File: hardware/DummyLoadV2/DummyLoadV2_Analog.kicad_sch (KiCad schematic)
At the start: 49 parts, among them J2 Conn_01x05, J5 Power, J8 Digital, Q1 FQP30N06L, Q2 2N7000, Q5 2N7000, U1 MAX4167, U2 LM4040-4.1, U3 MCP3302, U7 L78L05_TO92, U8 MCP4922

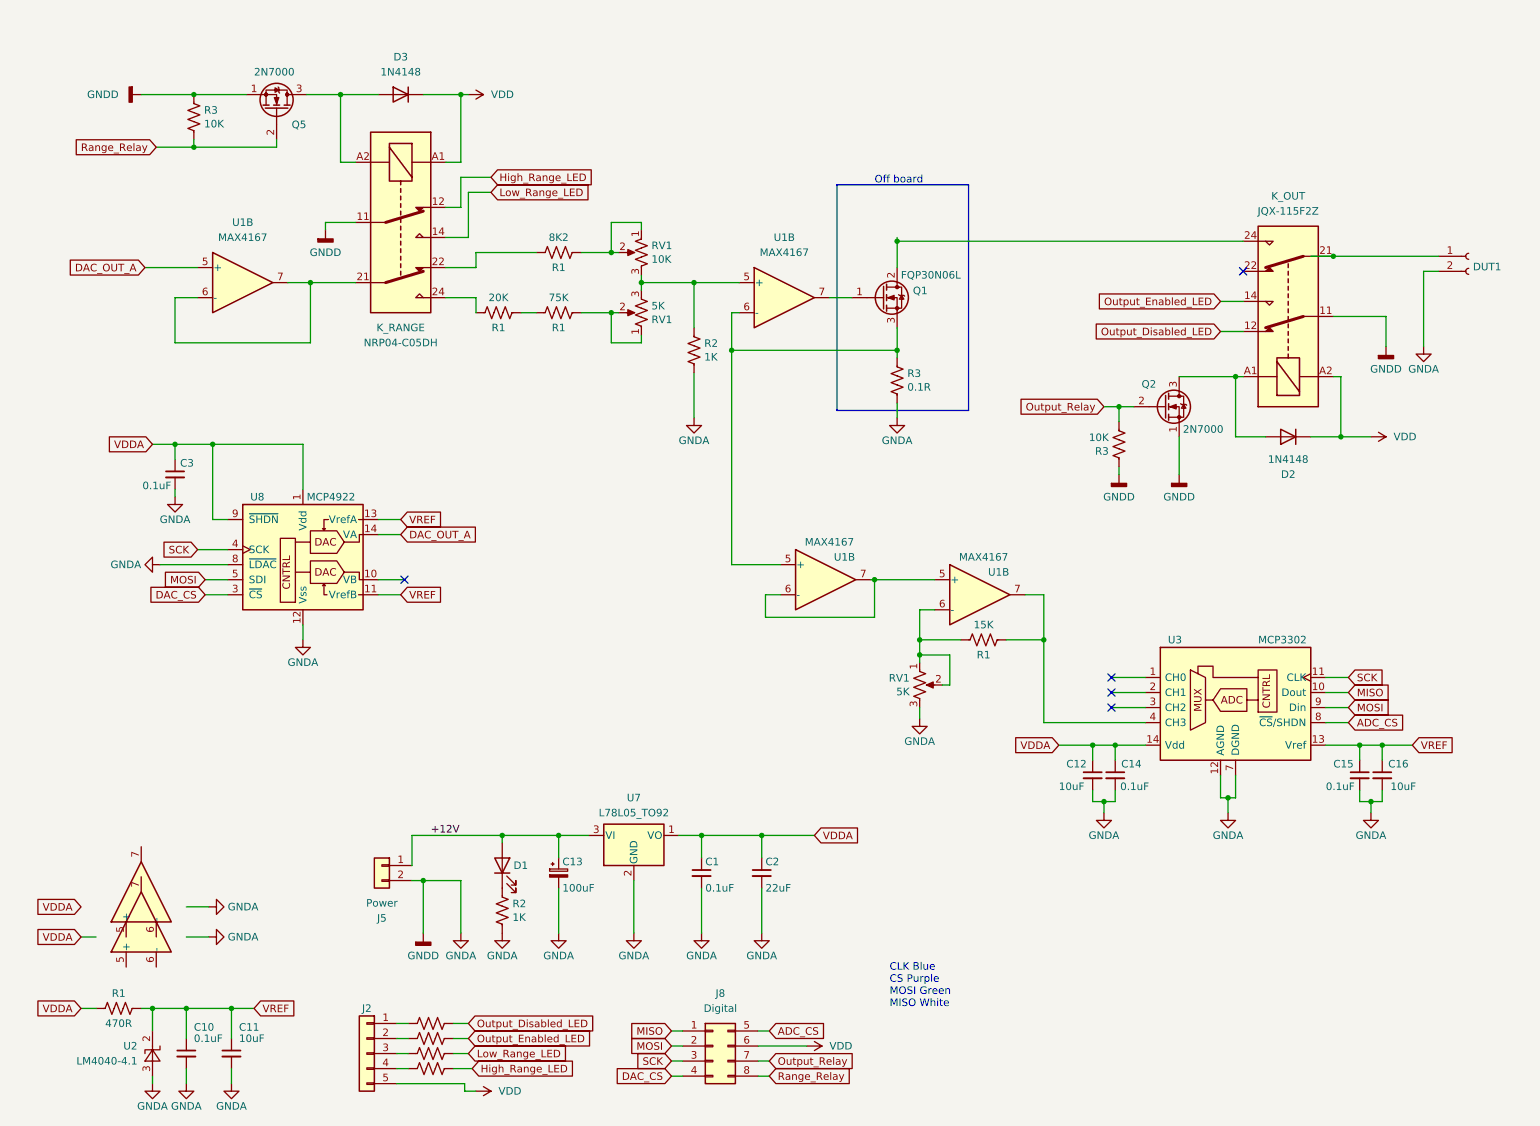
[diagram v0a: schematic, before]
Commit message: Updated schematic
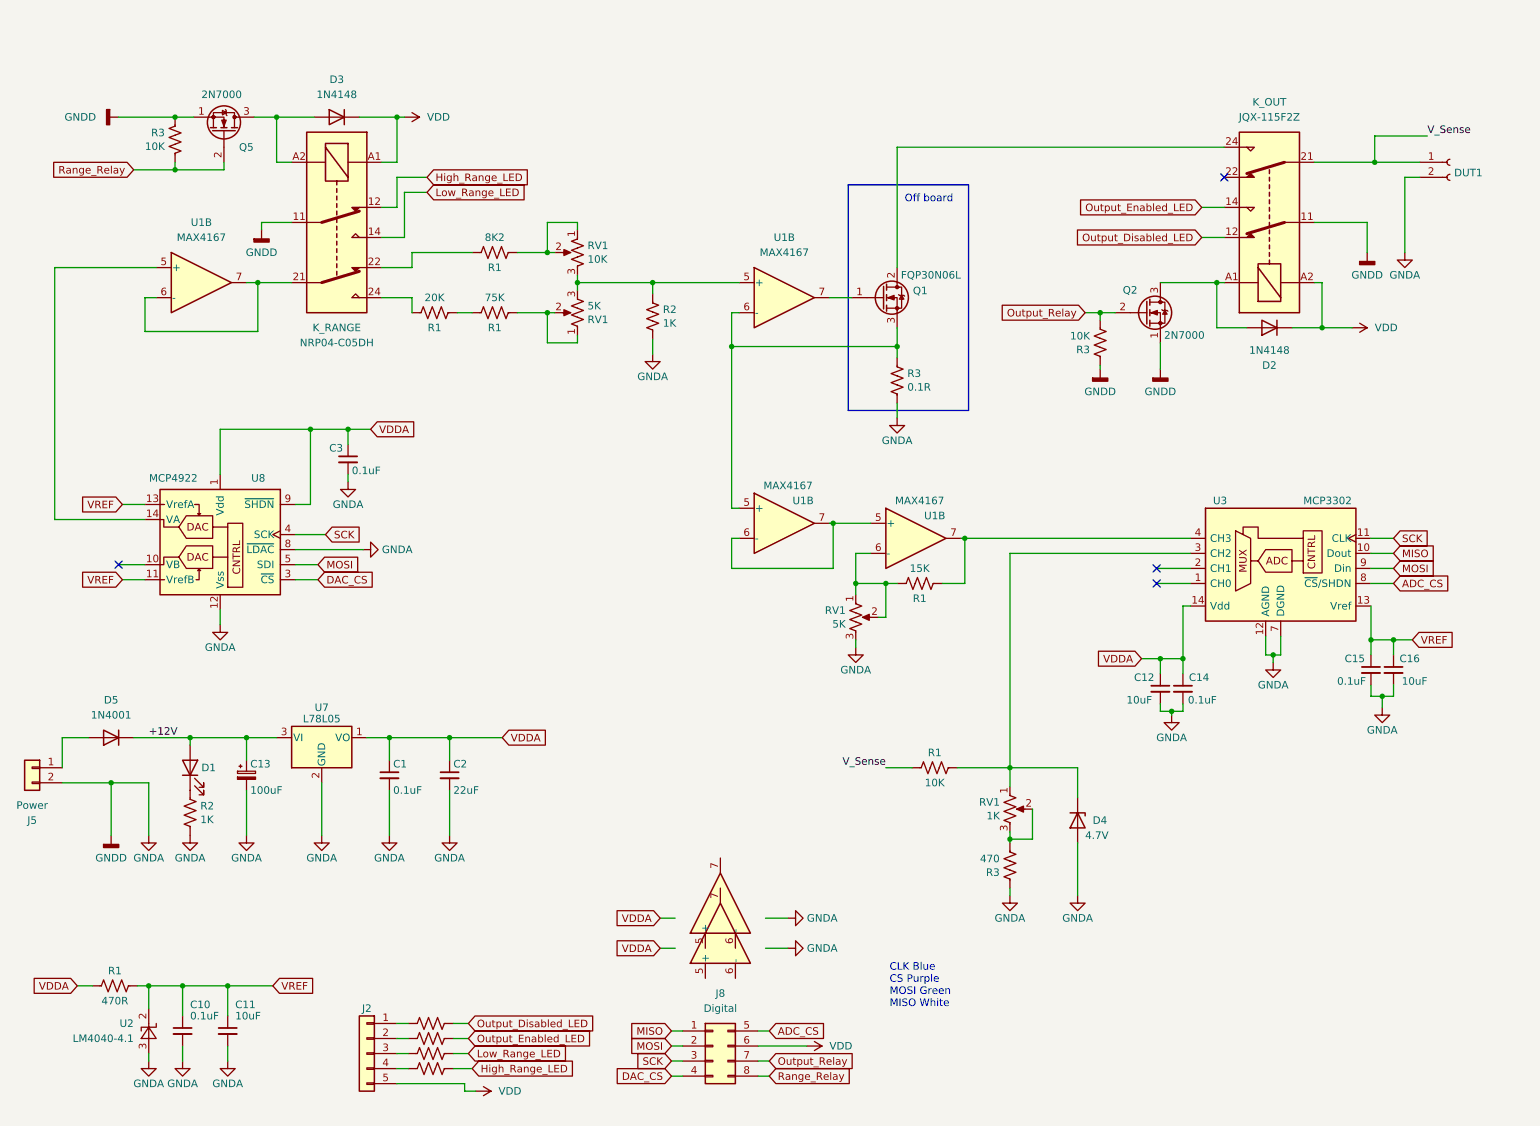
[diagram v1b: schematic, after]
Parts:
- added D4: 4.7V, symbol Device:D_Zener
- added D5: 1N4001, Diode_THT:D_DO-41_SOD81_P10.16mm_Horizontal, symbol Diode:1N4001
- added R1: 10K, symbol Device:R_US
- added R3: 470, symbol Device:R_US
- added RV1: 1K, symbol BasicDummyLoad-rescue:R_POT_US-Device
- U7: value L78L05_TO92 -> L78L05
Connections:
- net +12V: now also D5.1 (K); no longer J5.1 (Pin_1)
- net GNDA: now also D4.2 (A), R3.2
- net V_Sense: now reaches DUT1.1 (Pin_1), K_OUT.21
- net V_Sense: now also R1.2
- net at U3.3 (CH2): now also D4.1 (K), R1.1, RV1.1
- net DAC_OUT_A: no longer names the net of U1.5 (+), U8.14 (VA)
- new net: R3.1, RV1.2, RV1.3
- new net: D5.2 (A), J5.1 (Pin_1)
- no-connect marks 5 -> 4
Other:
- moved on the sheet: C1, C10, C11, C12, C13, C14, C15, C16, C2, C3, D1, D2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

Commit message: Updated schematic
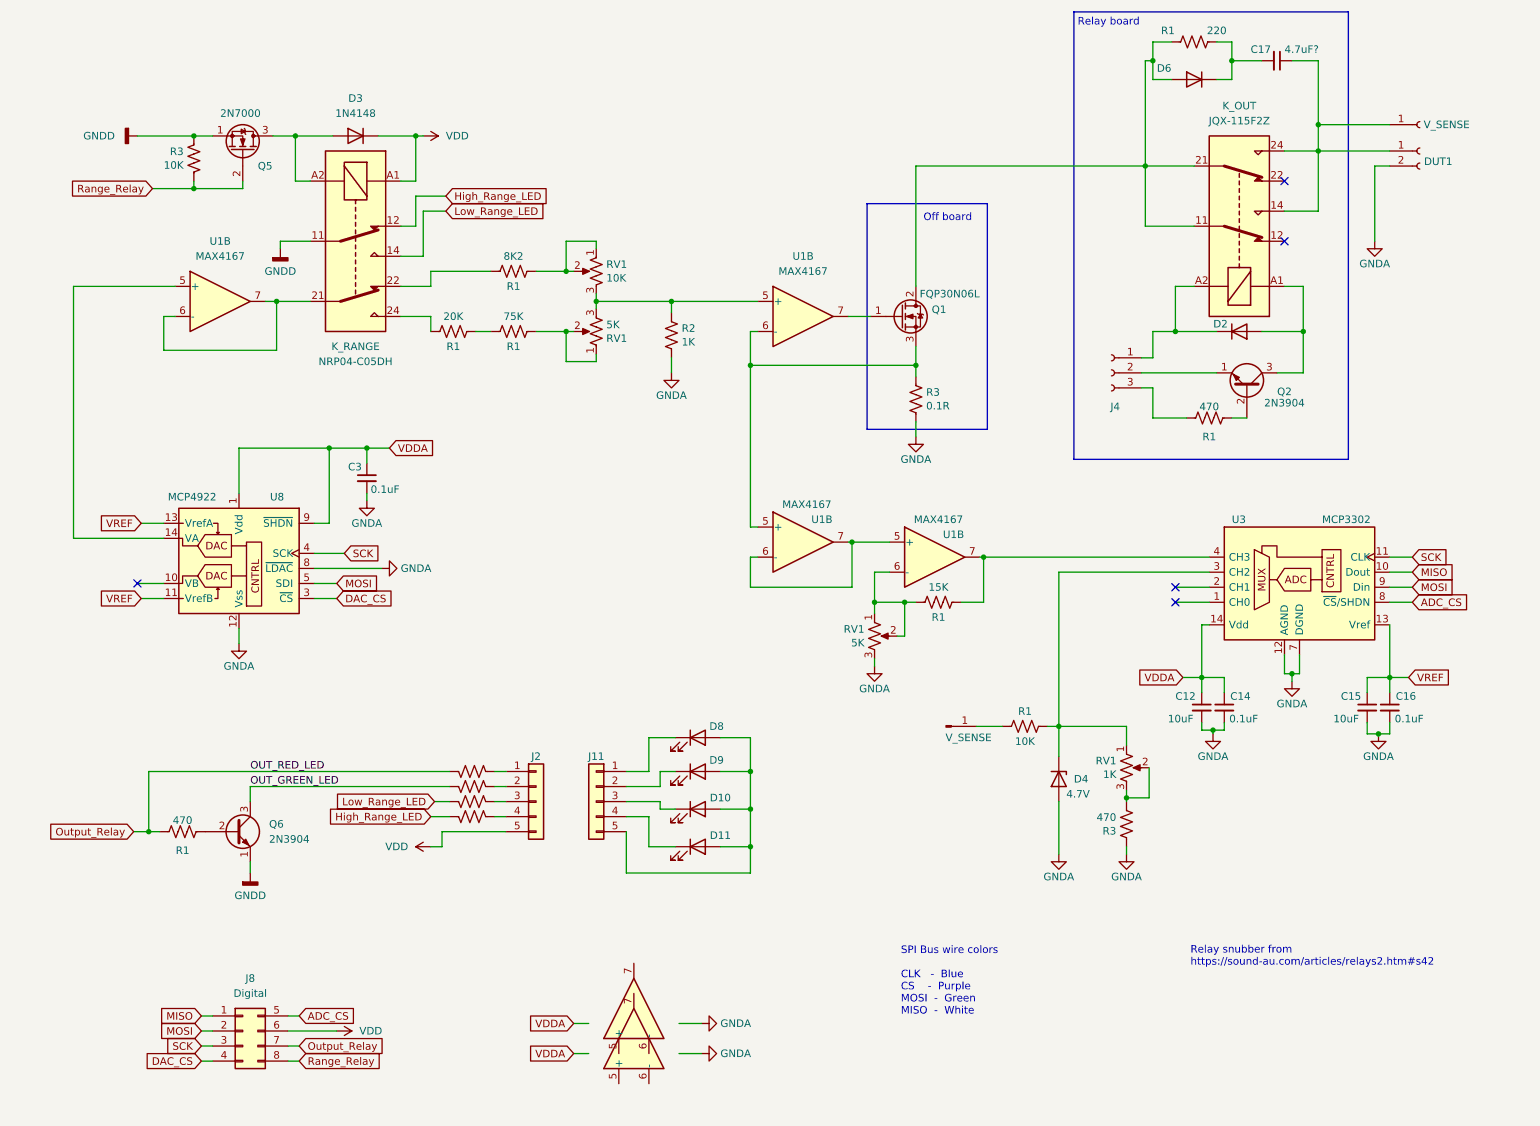
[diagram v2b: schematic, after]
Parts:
- removed C1, C10: 0.1uF, symbol Device:C_Small
- removed C11: 10uF, symbol Device:C_Small
- removed C13: 100uF, symbol Device:C_Polarized_Small
- removed C2: 22uF, symbol Device:C_Small
- removed D1: LED, symbol Device:LED
- removed D5: 1N4001, Diode_THT:D_DO-41_SOD81_P10.16mm_Horizontal, symbol Diode:1N4001
- removed J5: Power, symbol Connector_Generic:Conn_01x02
- removed Q2: 2N7000, Package_TO_SOT_THT:TO-92_Inline, symbol Transistor_FET:2N7000
- removed R1: 470R, symbol Device:R_US
- removed R2: 1K, symbol Device:R_US
- removed R3: 10K, symbol Device:R_US
- removed U2: LM4040-4.1, Package_TO_SOT_THT:TO-92_Inline, symbol Reference_Voltage:LM4040LP-4.1
- removed U7: L78L05, Package_TO_SOT_THT:TO-92_Inline, symbol Regulator_Linear:L78L05_TO92
- added C17: 4.7uF?, symbol Device:C_Small
- added D10, D11, D8, D9: LED, symbol Device:LED
- added D6: 1N4148, Diode_THT:D_DO-35_SOD27_P7.62mm_Horizontal, symbol Diode:1N4148
- added J11: Conn_01x05, symbol Connector_Generic:Conn_01x05
- added J4: Conn_01x03_Socket, symbol Connector:Conn_01x03_Socket
- added Q2, Q6: 2N3904, Package_TO_SOT_THT:TO-92_Inline, symbol Transistor_BJT:2N3904
- added R1 (x2): 470, symbol Device:R_US
- added R1: 220, symbol Device:R_US
- added V_SENSE: Conn_01x01_Pin, symbol Connector:Conn_01x01_Pin
- added V_SENSE: Conn_01x01_Socket, symbol Connector:Conn_01x01_Socket
- C15: value 0.1uF -> 10uF
- C16: value 10uF -> 0.1uF
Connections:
- net GNDA: no longer K_OUT.11, K_RANGE.11, Q5.1 (S), R3.2
- net Output_Relay: now also R1.1, R1.1
- net VDD: no longer D2.1 (K), K_OUT.A2
- net at D2.2 (A), K_OUT.A1: now also Q2.3 (C)
- net at K_OUT.24: now also DUT1.1 (Pin_1), K_OUT.14, C17.1, V_SENSE.1 (Pin_1); no longer Q1.2 (D)
- net Output_Disabled_LED: no longer names the net of K_OUT.12
- net Output_Disabled_LED: no longer R1.1
- net Output_Enabled_LED renamed OUT_GREEN_LED
- net OUT_GREEN_LED: now also Q6.3 (C); no longer K_OUT.14
- removed net V_Sense: DUT1.1 (Pin_1), K_OUT.21, R1.2
- new net: D8.1 (K), J11.1 (Pin_1)
- new net: D10.2 (A), D11.2 (A), D8.2 (A), D9.2 (A), J11.5 (Pin_5)
- new net: J4.2 (Pin_2), Q2.1 (E)
- new net: Q2.2 (B), R1.2
- new net: D9.1 (K), J11.2 (Pin_2)
- new net: D10.1 (K), J11.3 (Pin_3)
- new net: D11.1 (K), J11.4 (Pin_4)
- new net: R1.2, V_SENSE.1 (Pin_1)
- new net: C17.2, D6.1 (K), R1.2
- new net: D2.1 (K), J4.1 (Pin_1), K_OUT.A2
- new net: J4.3 (Pin_3), R1.1
- new net: D6.2 (A), K_OUT.11, K_OUT.21, Q1.2 (D), R1.1
- new net: Q6.2 (B), R1.2
- new net GNDD: K_RANGE.11, Q5.1 (S), Q6.1 (E), R3.2
- no-connect marks 4 -> 5
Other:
- note added: "Relay board"
- note added: "Relay snubber from https://sound-au.com/articles/relays2.htm#s42"
- note added: "SPI Bus wire colors CLK - Blue CS - Purple MOSI - Green MISO - White"
- note removed: "CLK Blue CS Purple MOSI Green MISO White"
- moved on the sheet: C12, C14, C15, C16, C3, D2, D3, DUT1, J2, J8, K_OUT, K_RANGE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
